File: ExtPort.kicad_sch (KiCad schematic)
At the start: 12 parts, among them J5 VE.Direct port (JST-PH 4), U7 SN74LVC1G125DBVR, U8 SN74LVC1G17DBVR

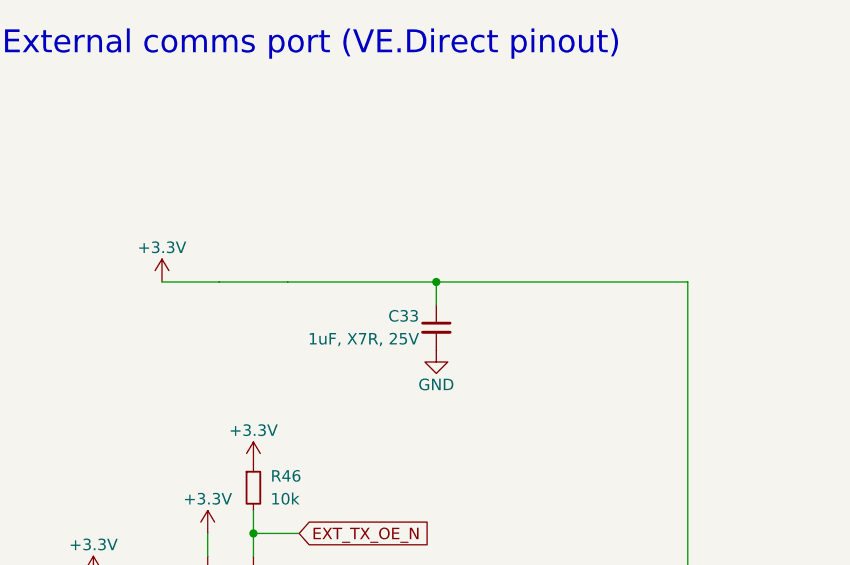
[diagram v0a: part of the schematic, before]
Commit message: Move power stage into its own PowerStage sheet; ExtPort, uC and PCB updates
Fugu2.kicad_sch: power stage moved out to the new hierarchical sheet
PowerStage.kicad_sch (sheet registered in Fugu2.kicad_pro). Includes the
staged ExtPort.kicad_sch and uC.kicad_sch edits, the PCB and a regenerated
Schematics.pdf.
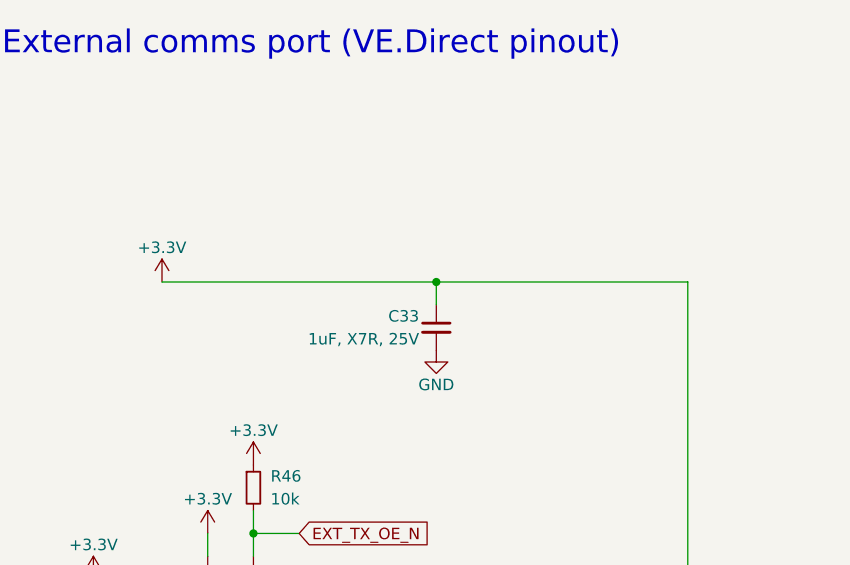
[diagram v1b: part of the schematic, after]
